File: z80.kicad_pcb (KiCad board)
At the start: 2 copper layers, 144.8 x 172.7 mm, 93 parts, among them J1 Conn_02x08_Odd_Even, J2 KMDGX-6S-BS, J3 Conn_02x20_Odd_Even, J5 USB_B, J6 PWR, SW1 KS01Q, U1 Z80CPU, U10 Z84C40, U11 SP232E, U12 SP232E, U13 74AHC541, U14 74AHC541, U15 Z84C20, U16 74AHC08, U17 Z84C30, U18 74HC164, U19 74HC164, U2 74AHC14, U3 SST39SF010, U4 74AHC32, U5 AS6C1008-55PCN, U6 74AHC138, U7 74AC574, U8 74AC574, U9 74AHC02, X1 ACH10MHZ, X2 1.8432MHz

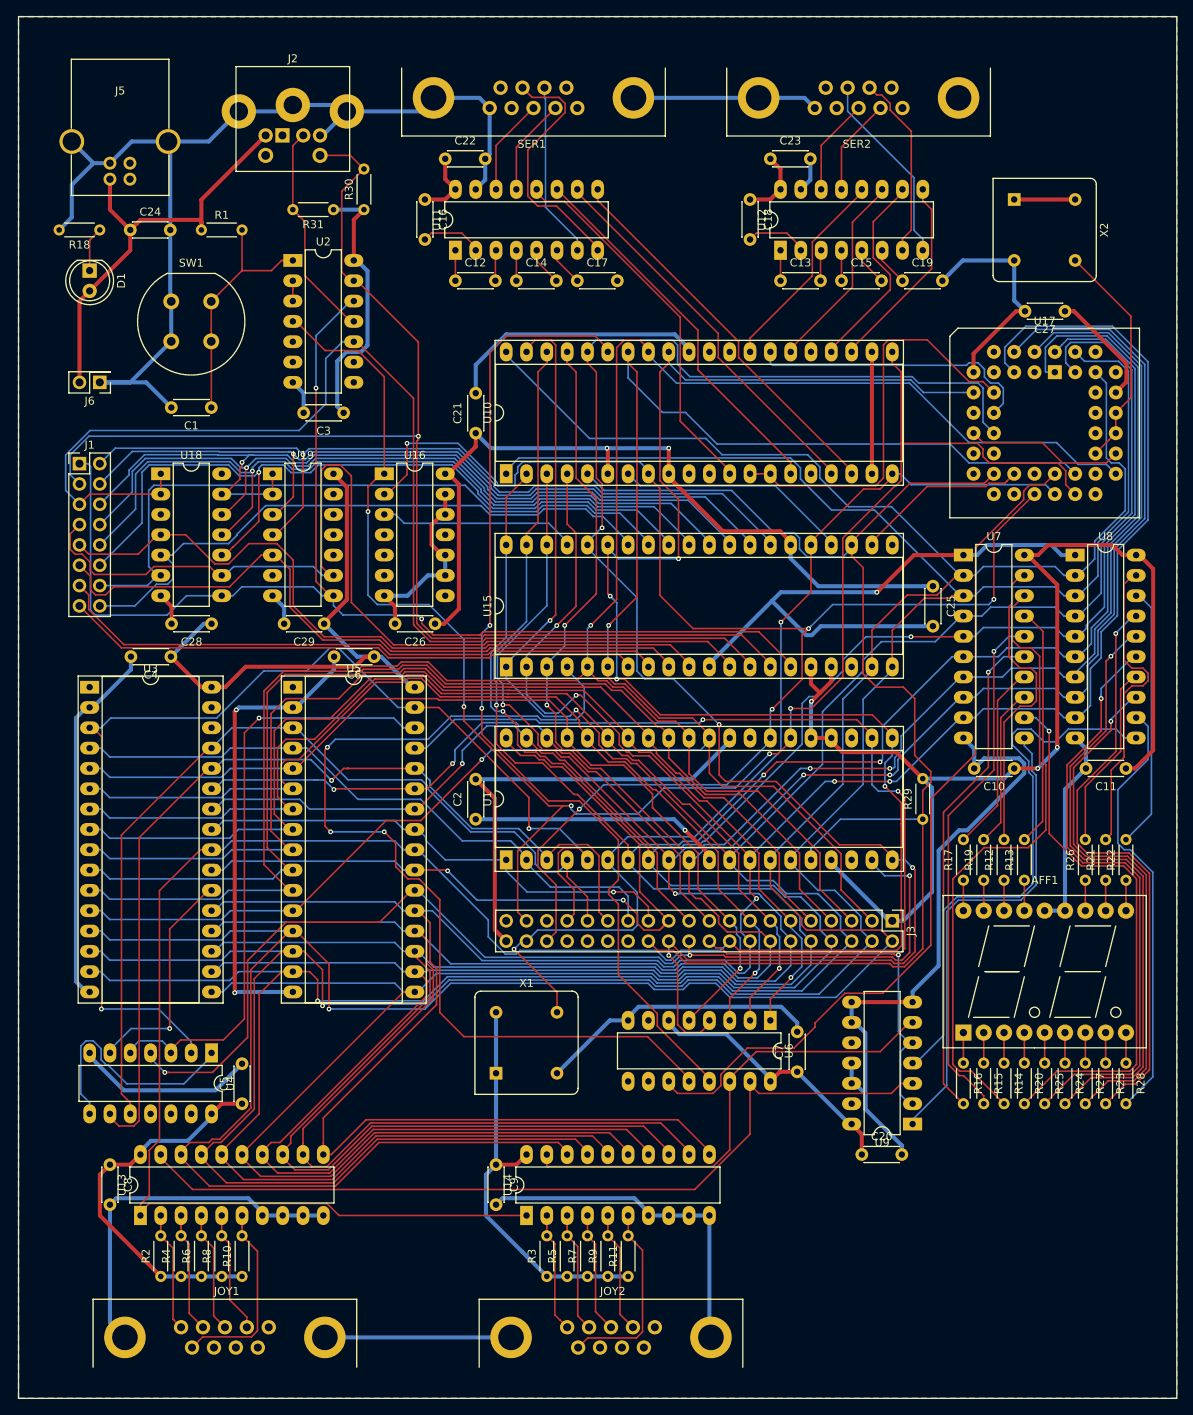
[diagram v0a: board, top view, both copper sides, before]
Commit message: Initial prototype PCB build.
git-svn-id: svn+ssh://dev.thehead.ca/depot/main/z80@619 995eaefb-0ce2-40e3-b8bc-69bf8729875b
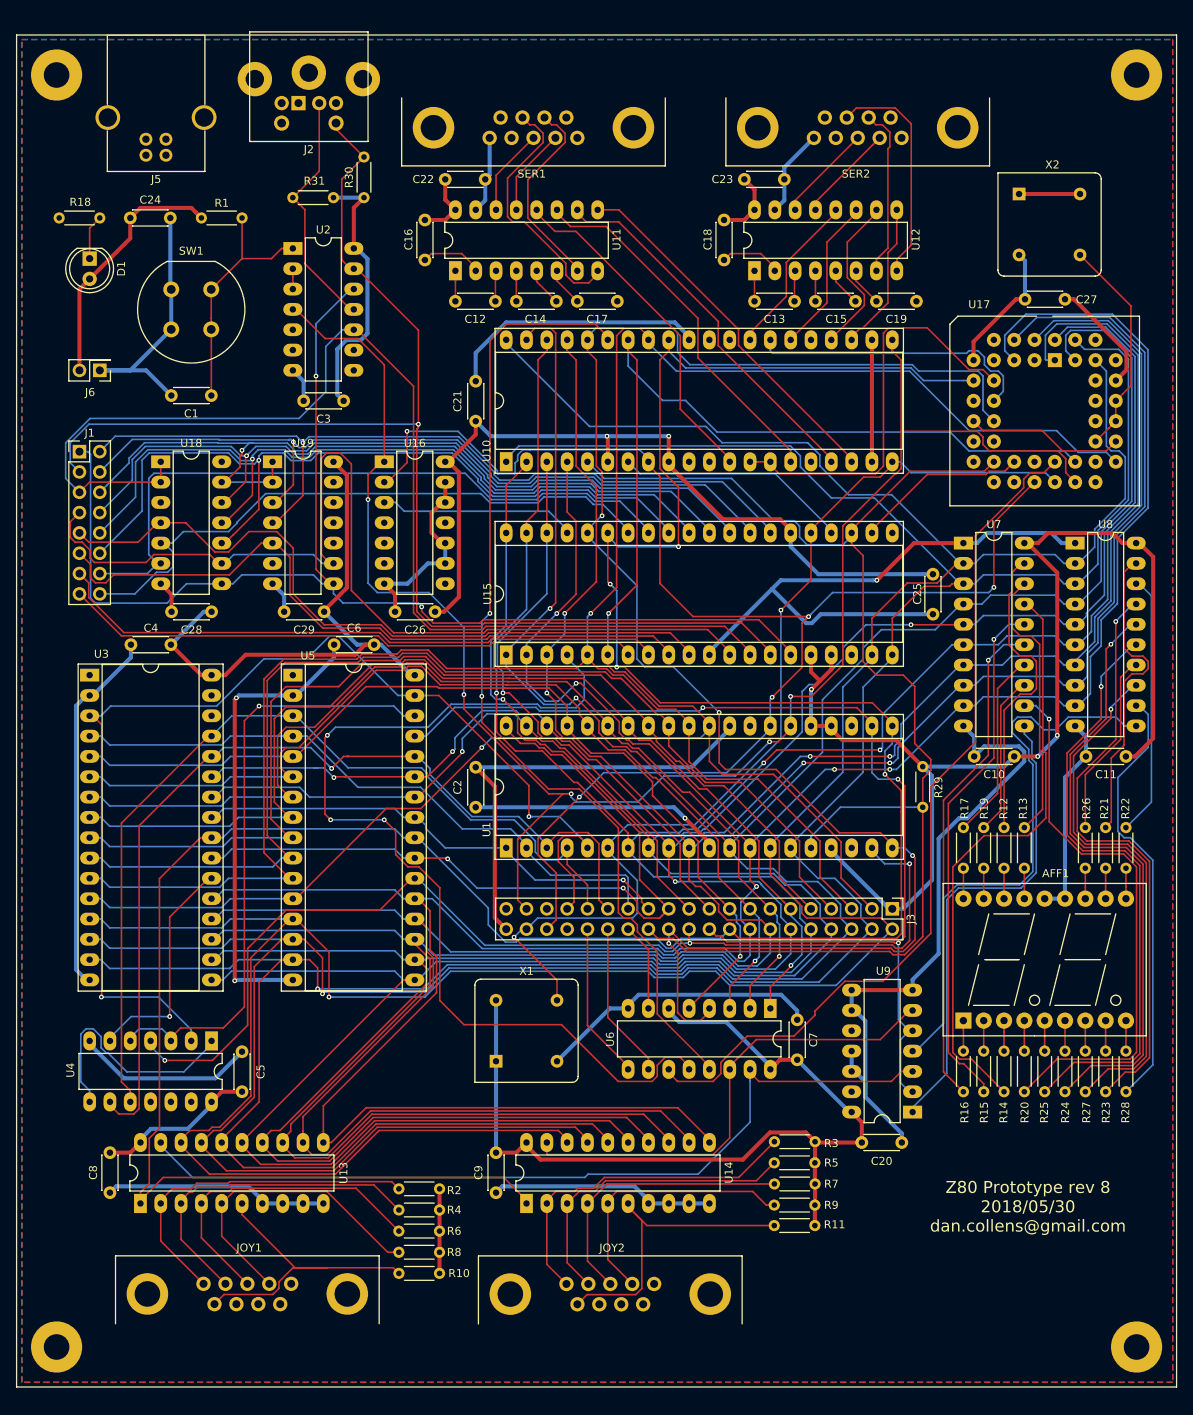
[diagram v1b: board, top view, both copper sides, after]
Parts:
- added REF**: MountingHole_3.2mm_M3_Pad, Mounting_Holes:MountingHole_3.2mm_M3_Pad, F.Cu at (20.0, 20.0)
- added REF**: MountingHole_3.2mm_M3_Pad, Mounting_Holes:MountingHole_3.2mm_M3_Pad, F.Cu at (20.0, 179.0)
- added REF**: MountingHole_3.2mm_M3_Pad, Mounting_Holes:MountingHole_3.2mm_M3_Pad, F.Cu at (155.0, 179.0)
- added REF**: MountingHole_3.2mm_M3_Pad, Mounting_Holes:MountingHole_3.2mm_M3_Pad, F.Cu at (155.0, 20.0)
- moved R3 37.5 mm to (114.8, 153.3), turned to 180 degrees
- moved R2 36.5 mm to (67.9, 159.2), turned to 180 degrees
- moved R5 34.1 mm to (114.8, 156.0), turned to 180 degrees
- moved R4 33.4 mm to (67.9, 161.9), turned to 180 degrees
- moved R7 30.7 mm to (114.8, 158.6), turned to 180 degrees
- moved R6 30.3 mm to (67.9, 164.5), turned to 180 degrees
- moved R8 27.4 mm to (67.9, 167.2), turned to 180 degrees
- moved R9 27.4 mm to (114.8, 161.3), turned to 180 degrees
- moved R10 24.7 mm to (67.9, 169.8), turned to 180 degrees
- moved R11 24.2 mm to (114.8, 163.8), turned to 180 degrees
- moved JOY1 6.11 mm to (38.4, 171.1)
- moved JOY2 5.41 mm to (83.7, 171.1)
- moved J5 5.40 mm to (31.2, 30.0)
- moved J2 4.51 mm to (51.5, 15.0)
- moved C18 4.14 mm to (103.4, 38.1)
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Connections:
- J3 pad 28: (no net) -> /~IORQ7
- J3 pad 30: (no net) -> /~IORQ5
- J3 pad 32: (no net) -> /~IORQ6
- U6 pad 10: (no net) -> /~IORQ5
- U6 pad 7: (no net) -> /~IORQ7
- U6 pad 9: (no net) -> /~IORQ6
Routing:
- net GND: track 786.4 -> 617.9 mm
- net Net-(JOY1-Pad1): track 15.0 -> 43.8 mm
- net Net-(JOY2-Pad1): track 15.0 -> 43.0 mm
- net Net-(JOY1-Pad2): track 15.1 -> 42.1 mm
- net Net-(JOY1-Pad3): track 15.2 -> 40.4 mm
- net Net-(JOY2-Pad2): track 15.1 -> 39.1 mm
- net Net-(JOY1-Pad4): track 15.3 -> 38.4 mm
- net Net-(JOY2-Pad3): track 15.2 -> 35.6 mm
- net /~IORQ6: track 0.00 -> 19.6 mm
- net /~IORQ5: track 0.00 -> 19.6 mm
- net Net-(JOY2-Pad4): track 15.3 -> 33.7 mm
- net Net-(JOY1-Pad6): track 24.7 -> 40.5 mm
- net Net-(JOY2-Pad6): track 24.6 -> 39.5 mm
- net VCC: track 618.0 -> 605.4 mm
- net /~IORQ7: track 0.00 -> 11.0 mm
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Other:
- board size 144.8 x 172.7 mm -> 145 x 169 mm
- board text added: "Z80 Prototype rev 8 2018/05/30 dan.collens@gmail.com"
